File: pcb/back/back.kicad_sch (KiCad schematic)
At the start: 59 parts, among them J1 Conn_01x02, J2 USB_B_Micro, U1 ATSAMD21G18A-A, U2 LSM6DS3, U3 XC6206PxxxMR, U4 TP4057

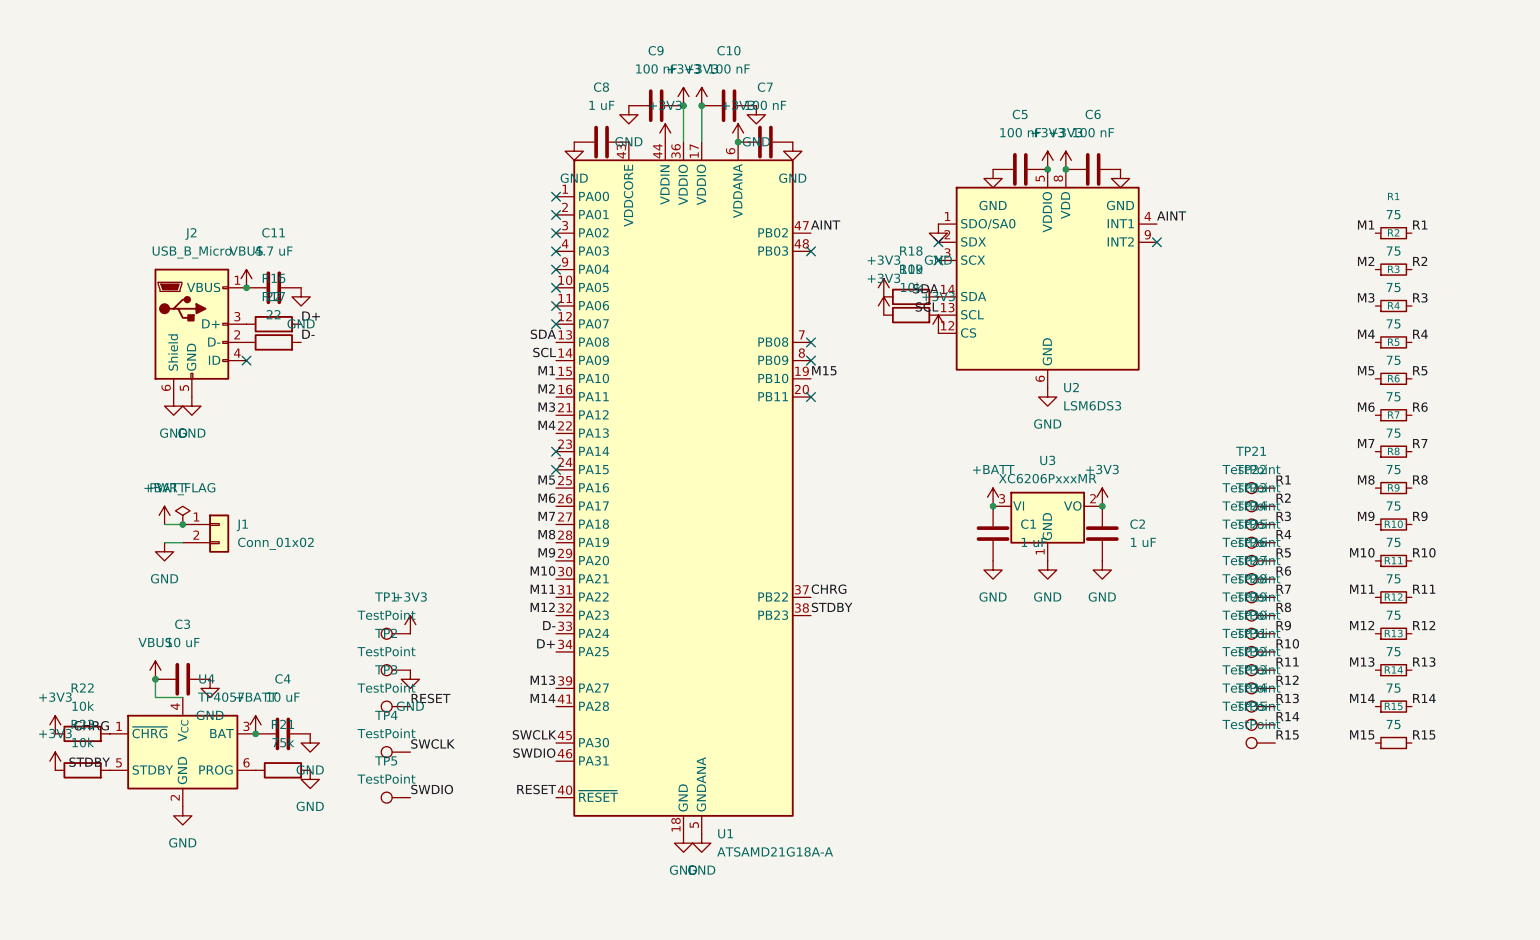
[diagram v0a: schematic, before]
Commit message: Update accelerometer
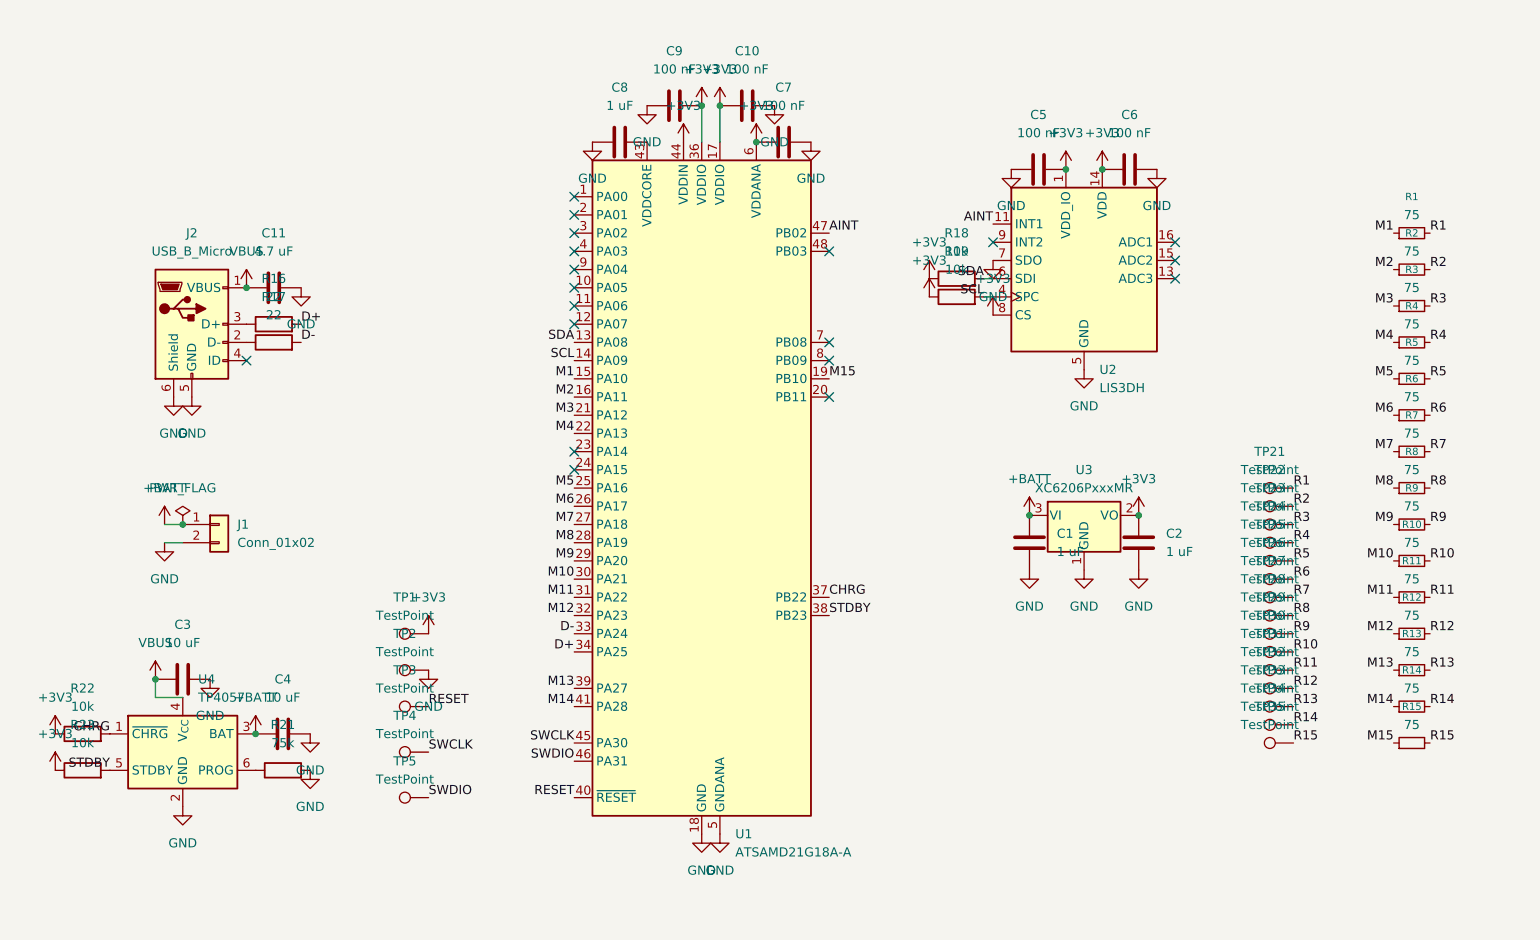
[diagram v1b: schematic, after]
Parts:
- removed U2: LSM6DS3, Package_LGA:LGA-14_3x2.5mm_P0.5mm_LayoutBorder3x4y, symbol Sensor_Motion:LSM6DS3
- added U2: LIS3DH, Package_LGA:LGA-16_3x3mm_P0.5mm_LayoutBorder3x5y, symbol Sensor_Motion:LIS3DH
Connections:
- net +3V3: now also U2.1 (VDD_IO), U2.14 (VDD), U2.8 (CS)
- net AINT: now also U2.11 (INT1)
- net GND: now also U2.10 (GND), U2.12 (GND), U2.5 (GND), U2.7 (SDO)
- net SCL: now also U2.4 (SPC)
- net SDA: now also U2.6 (SDI)
- no-connect marks 18 -> 19
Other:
- moved on the sheet: C1, C10, C2, C5, C6, C7, C8, C9, R1, R10, R11, R12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

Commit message: Format schematics
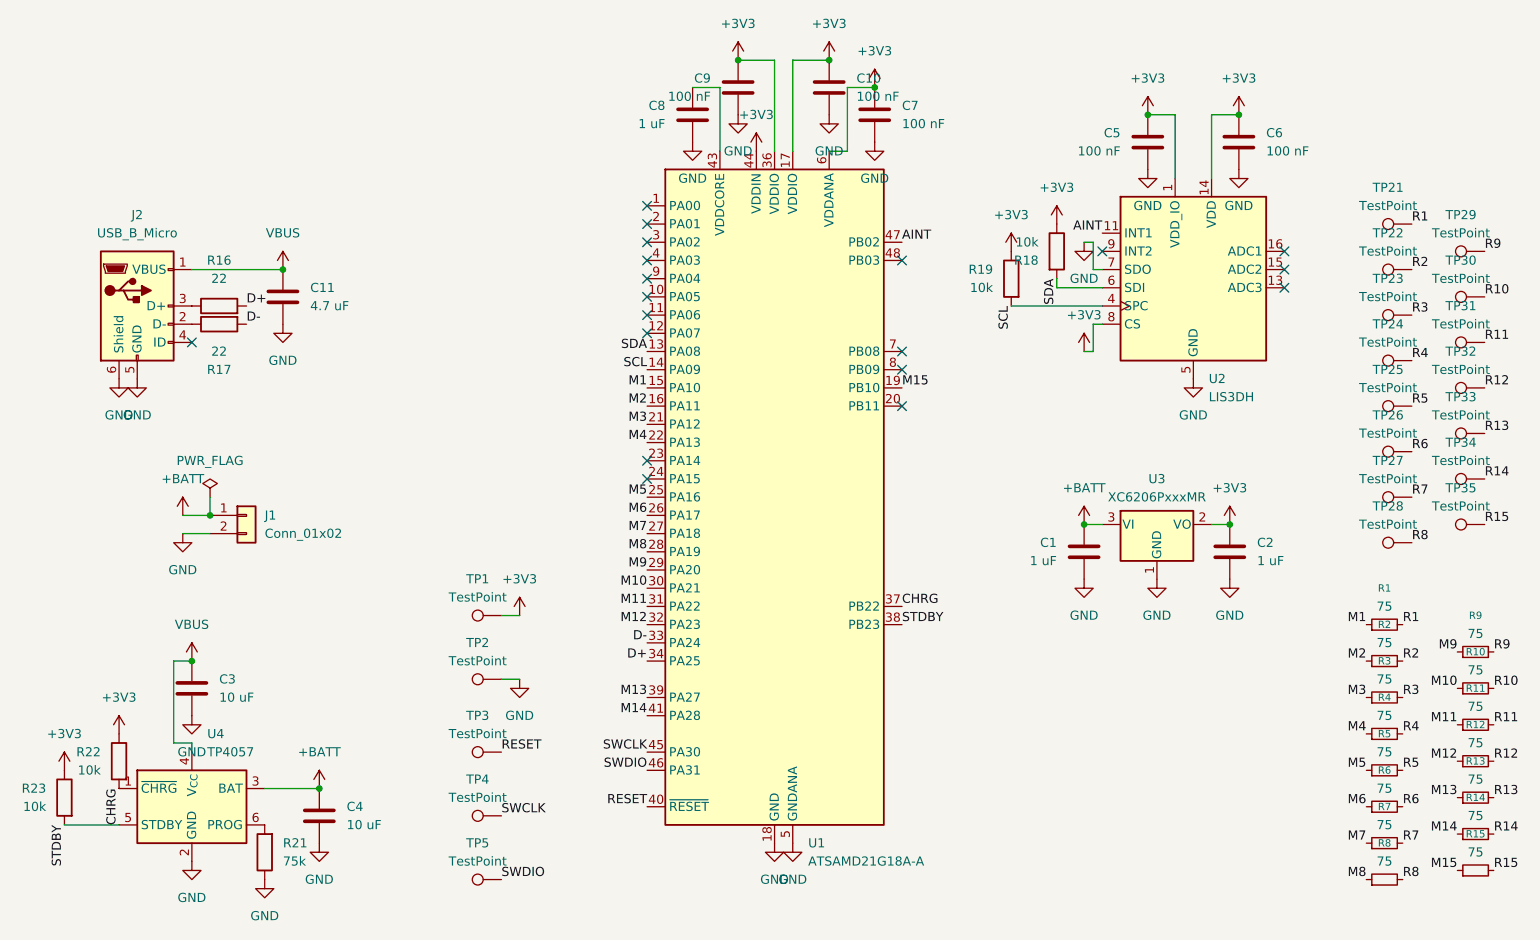
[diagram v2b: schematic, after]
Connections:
- net +3V3: now also C10.2, C6.2; no longer C10.1, C6.1
- net +BATT: now also C4.1; no longer C4.2
- net GND: now also C10.1, C11.1, C3.2, C4.2, C6.1, C8.2, R21.1; no longer C10.2, C11.2, C3.1, C4.1, C6.2, C8.1, R21.2
- net VBUS: now also C11.2, C3.1; no longer C11.1, C3.2
- net at U4.6 (PROG): now also R21.2; no longer R21.1
- net at U1.43 (VDDCORE): now also C8.1; no longer C8.2
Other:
- moved on the sheet: C1, C10, C11, C2, C3, C4, C5, C6, C7, C8, C9, J1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
